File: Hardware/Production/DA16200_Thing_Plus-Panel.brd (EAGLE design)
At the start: 112.3 x 207 mm, 1530 parts, among them J1 Qwiic, J10 CORTEX_JTAG_DEBUG_PTH_NS, J11 Qwiic, J13 USB C, J14 THING_PLUS, J15 CORTEX_JTAG_DEBUG_PTH_NS, J16 Qwiic, J18 USB C, J19 THING_PLUS, J2 THING_PLUS, J20 CORTEX_JTAG_DEBUG_PTH_NS, J21 Qwiic, J23 USB C, J24 THING_PLUS, J25 CORTEX_JTAG_DEBUG_PTH_NS, J26 Qwiic, J28 USB C, J29 THING_PLUS, J3 Qwiic, J30 CORTEX_JTAG_DEBUG_PTH_NS, J31 Qwiic, J33 USB C, J34 THING_PLUS, J35 CORTEX_JTAG_DEBUG_PTH_NS, J36 Qwiic, J38 USB C, J39 THING_PLUS, J40 CORTEX_JTAG_DEBUG_PTH_NS, J41 Qwiic, J43 USB C, J44 THING_PLUS, J45 CORTEX_JTAG_DEBUG_PTH_NS, J46 Qwiic, J48 USB C, J49 THING_PLUS, J5 USB C, J50 CORTEX_JTAG_DEBUG_PTH_NS, J51 Qwiic, J53 USB C, J54 THING_PLUS, J55 CORTEX_JTAG_DEBUG_PTH_NS, J56 Qwiic, J58 USB C, J59 THING_PLUS, J60 CORTEX_JTAG_DEBUG_PTH_NS, J7 CORTEX_JTAG_DEBUG_PTH_NS, J8 USB C, J9 THING_PLUS, Q1 20V/4.2A/52mΩ/1.4W, Q10 20V/4.2A/52mΩ/1.4W, Q11 20V/4.2A/52mΩ/1.4W, Q12 20V/4.2A/52mΩ/1.4W, Q2 20V/4.2A/52mΩ/1.4W, Q3 20V/4.2A/52mΩ/1.4W, Q4 20V/4.2A/52mΩ/1.4W, Q5 20V/4.2A/52mΩ/1.4W, Q6 20V/4.2A/52mΩ/1.4W, Q7 20V/4.2A/52mΩ/1.4W, Q8 20V/4.2A/52mΩ/1.4W, Q9 20V/4.2A/52mΩ/1.4W, U1 DA16200MOD, U10 MCP73831, U11 DA16200MOD, U12 CH340E_MSOP10, U13 XC6222B331MR-G, U14 MCP73831, U15 DA16200MOD, U16 CH340E_MSOP10, U17 XC6222B331MR-G, U18 MCP73831, U19 DA16200MOD, U2 CH340E_MSOP10, U20 CH340E_MSOP10, U21 XC6222B331MR-G, U22 MCP73831, U23 DA16200MOD, U24 CH340E_MSOP10, U25 XC6222B331MR-G, U26 MCP73831, U27 DA16200MOD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

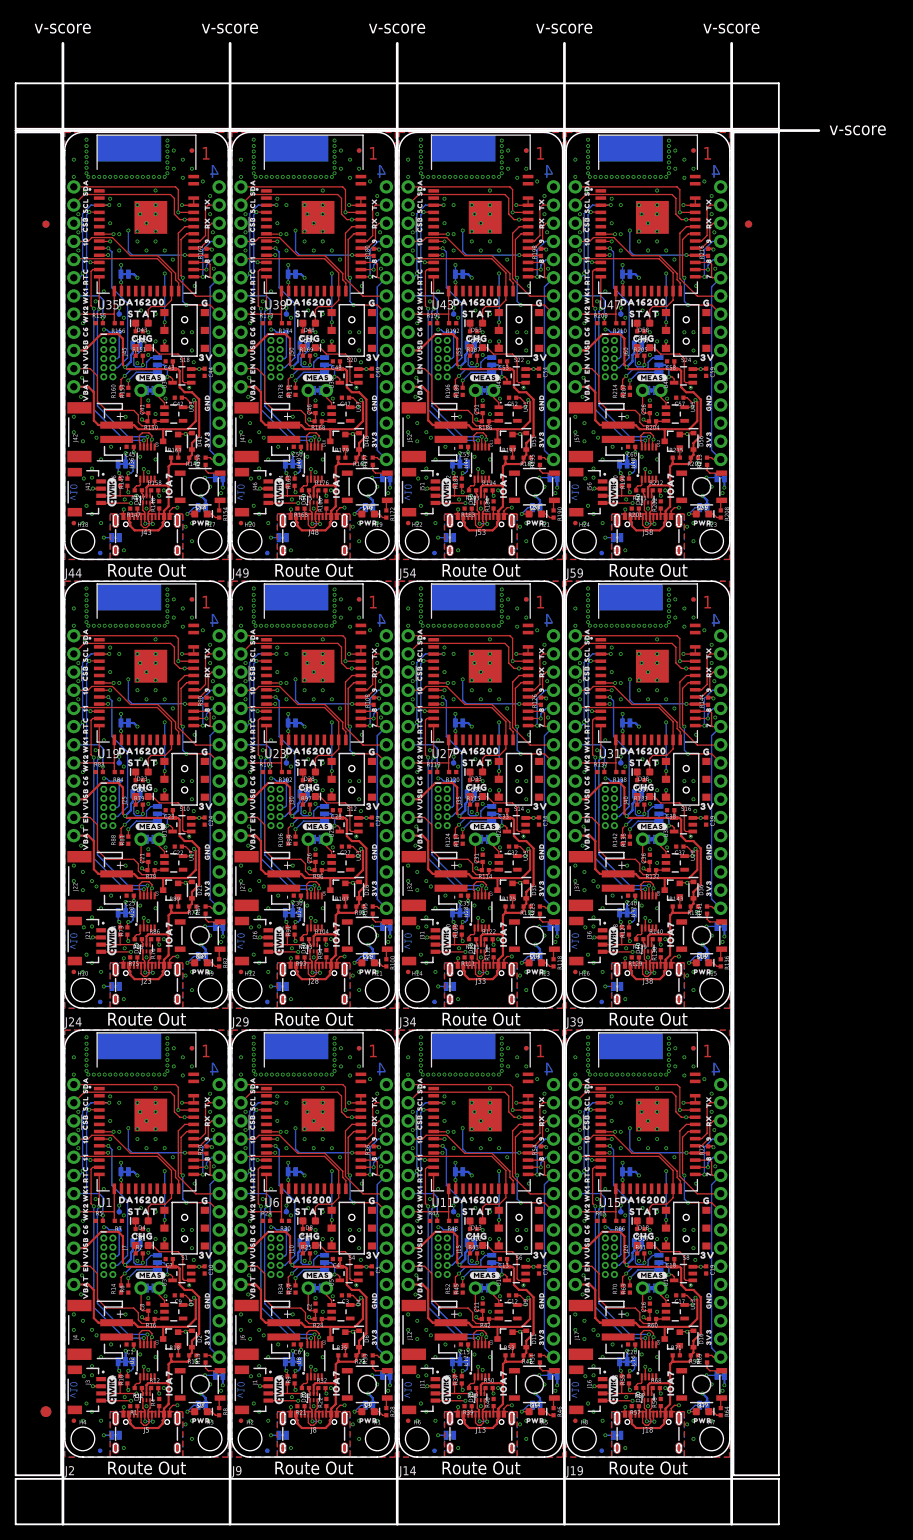
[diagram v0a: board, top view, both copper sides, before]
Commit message: Update production files
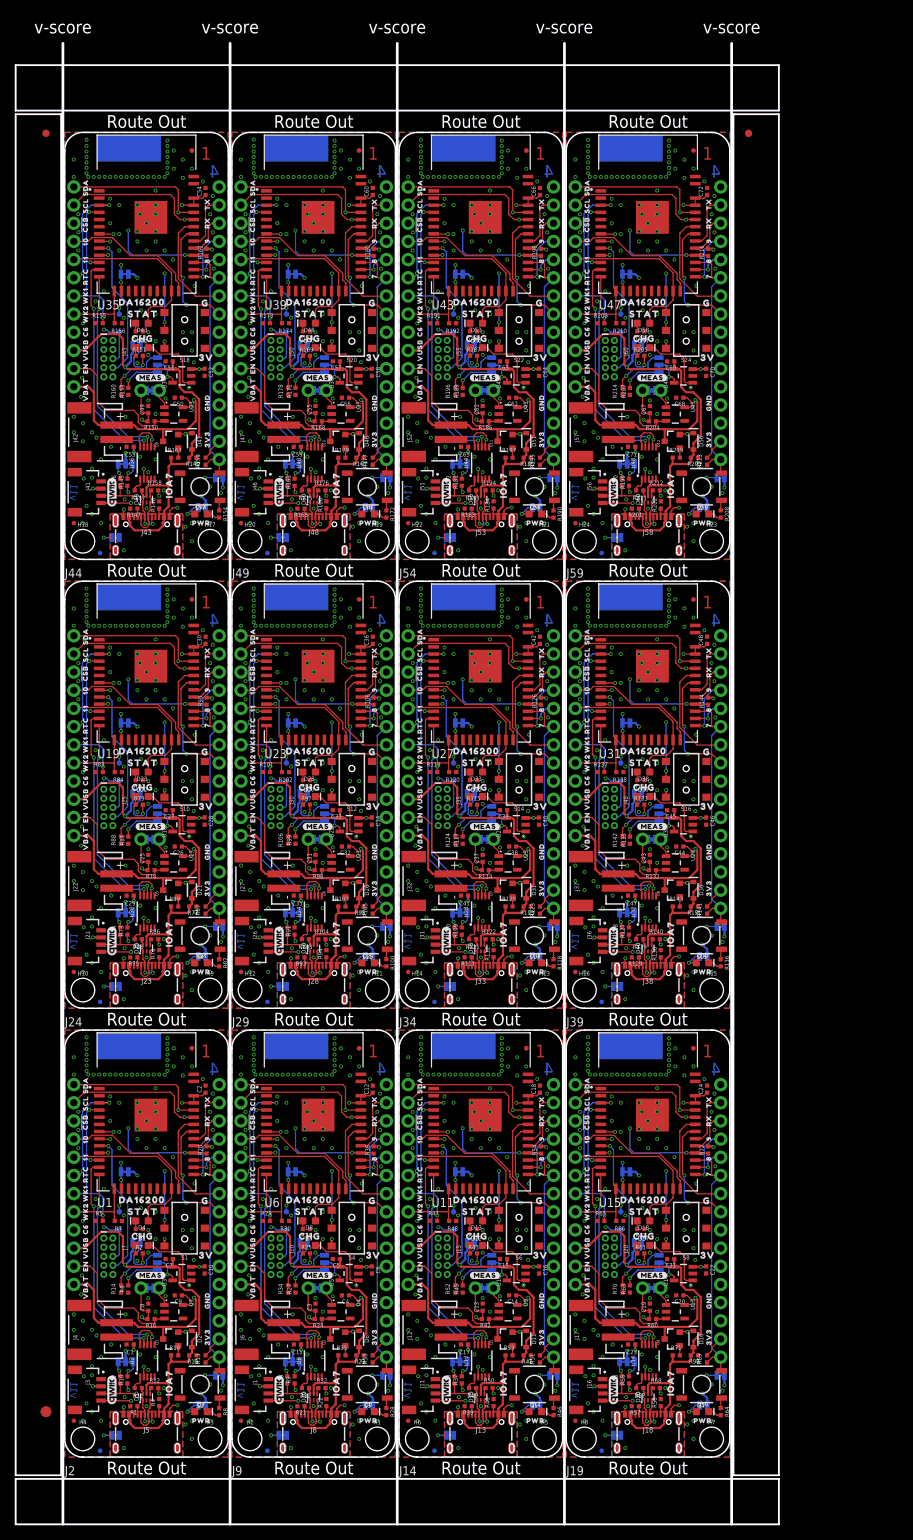
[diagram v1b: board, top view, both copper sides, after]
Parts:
- added C61, C67: 1.0uF, SparkFun-Capacitors:0402-TIGHT
- added C62, C68: 2.2uF, SparkFun-Capacitors:0402-TIGHT
- added C63, C64, C69, C70: 4.7uF, SparkFun-Capacitors:0402-TIGHT
- added C65, C66, C71, C72: 0.1uF, SparkFun-Capacitors:0402-TIGHT
- C11, C2, C36, C41: value 1.0uF -> 0.1uF
- C12, C17, C42, C47: value 2.2uF -> 0.1uF
- C13, C19, C43, C49: value 4.7uF -> 1.0uF
- C14, C38, C4, C44: value 4.7uF -> 2.2uF
- C15, C40, C45, C6: value 0.1uF -> 4.7uF
- C16, C21, C46, C51: value 1.0uF -> 4.7uF
- C18, C23, C24, C29, C48, C53, C54, C59: value 4.7uF -> 0.1uF
- C20, C50: value 0.1uF -> 2.2uF
- C22, C27, C52, C57: value 2.2uF -> 4.7uF
- C25, C55: value 0.1uF -> 1.0uF
- C26, C56: value 1.0uF -> 2.2uF
- C3, C37: value 2.2uF -> 1.0uF
- R105, R123, R13, R141, R159, R177, R195, R213, R33, R51, R69, R87: value 200 -> 10k
- moved C23 98.8 mm to (79.2, 15.7)
- moved C43 96.6 mm to (81.8, 83.7), turned to 90 degrees
- moved C22 94.6 mm to (89.7, 26.2), turned to 270 degrees
- moved C44 93.8 mm to (86.0, 85.3), turned to 180 degrees
- moved C21 92.0 mm to (84.7, 27.7), turned to 180 degrees
- moved C45 91.1 mm to (84.7, 90.4)
- moved C41 81.1 mm to (55.9, 78.5), turned to 180 degrees
- moved C47 80.3 mm to (79.2, 78.5)
- moved C24 79.6 mm to (89.8, 51.4), turned to 90 degrees
- moved C46 79.3 mm to (89.7, 88.9), turned to 270 degrees
- moved C48 64.8 mm to (89.8, 114.2), turned to 90 degrees
- moved C42 60.9 mm to (66.4, 114.2), turned to 90 degrees
- moved C59 58.1 mm to (32.5, 141.2), turned to 180 degrees
- moved C53 53.5 mm to (9.14, 141.2)
- moved C54 53.0 mm to (19.7, 176.9), turned to 90 degrees
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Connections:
- removed net N$107 (its old number): DA_MEAS3.1, U15.15, U15.34, U15.35
- removed net N$117 (its old number): C21.1, D21.C, MEAS4.1, MEAS4.3, Q5.2, R78.2
- removed net N$126 (its old number): R87.1, S9.3
- removed net N$134 (its old number): DA_MEAS4.1, U19.15, U19.34, U19.35
- removed net N$144 (its old number): C26.1, D26.C, MEAS5.1, MEAS5.3, Q6.2, R96.2
- removed net N$153: R105.1, S11.3
- removed net N$161 (its old number): DA_MEAS5.1, U23.15, U23.34, U23.35
- removed net N$171 (its old number): C31.1, D31.C, MEAS6.1, MEAS6.3, Q7.2, R114.2
- removed net N$180 (its old number): R123.1, S13.3
- removed net N$188 (its old number): DA_MEAS6.1, U27.15, U27.34, U27.35
- removed net N$198 (its old number): C36.1, D36.C, MEAS7.1, MEAS7.3, Q8.2, R132.2
- removed net N$215 (its old number): DA_MEAS7.1, U31.15, U31.34, U31.35
- removed net N$225 (its old number): C41.1, D41.C, MEAS8.1, MEAS8.3, Q9.2, R150.2
- removed net N$234 (its old number): R159.1, S17.3
- removed net N$242 (its old number): DA_MEAS8.1, U35.15, U35.34, U35.35
- removed net N$252 (its old number): C46.1, D46.C, MEAS9.1, MEAS9.3, Q10.2, R168.2
- removed net N$261 (its old number): R177.1, S19.3
- removed net N$279 (its old number): C51.1, D51.C, MEAS10.1, MEAS10.3, Q11.2, R186.2
- removed net N$288 (its old number): R195.1, S21.3
- removed net N$296 (its old number): DA_MEAS10.1, U43.15, U43.34, U43.35
- removed net N$306 (its old number): C56.1, D56.C, MEAS11.1, MEAS11.3, Q12.2, R204.2
- removed net N$315: R213.1, S23.3
- removed net N$323: DA_MEAS11.1, U47.15, U47.34, U47.35
- removed net N$36 (its old number): C2.1, D6.C, MEAS1.1, MEAS1.3, Q2.2, R24.2
- removed net N$45 (its old number): R33.1, S3.3
- removed net N$53 (its old number): DA_MEAS1.1, U6.15, U6.34, U6.35
- removed net N$63 (its old number): C11.1, D11.C, MEAS2.1, MEAS2.3, Q3.2, R42.2
- removed net N$72 (its old number): R51.1, S5.3
- removed net N$8 (its old number): R13.1, S2.3
- removed net N$80 (its old number): DA_MEAS2.1, U11.15, U11.34, U11.35
- removed net N$90 (its old number): C16.1, D16.C, MEAS3.1, MEAS3.3, Q4.2, R60.2
- removed net N$99 (its old number): R69.1, S7.3
- new net N$103: C24.1, DA_MEAS3.1, U15.15, U15.34, U15.35
- new net N$113: C25.1, D21.C, MEAS4.1, MEAS4.3, Q5.2, R78.2
- new net N$129: C30.1, DA_MEAS4.1, U19.15, U19.34, U19.35
- new net N$139: C31.1, D26.C, MEAS5.1, MEAS5.3, Q6.2, R96.2
- new net N$155: C36.1, DA_MEAS5.1, U23.15, U23.34, U23.35
- new net N$165: C37.1, D31.C, MEAS6.1, MEAS6.3, Q7.2, R114.2
- new net N$181: C42.1, DA_MEAS6.1, U27.15, U27.34, U27.35
- new net N$191: C43.1, D36.C, MEAS7.1, MEAS7.3, Q8.2, R132.2
- new net N$217: C49.1, D41.C, MEAS8.1, MEAS8.3, Q9.2, R150.2
- new net N$233: C54.1, DA_MEAS8.1, U35.15, U35.34, U35.35
- new net N$243: C55.1, D46.C, MEAS9.1, MEAS9.3, Q10.2, R168.2
- new net N$259: C60.1, DA_MEAS9.1, U39.15, U39.34, U39.35
- new net N$285: C66.1, DA_MEAS10.1, U43.15, U43.34, U43.35
- new net N$295: C67.1, D56.C, MEAS11.1, MEAS11.3, Q12.2, R204.2
- new net N$311: C72.1, DA_MEAS11.1, U47.15, U47.34, U47.35
- new net N$35: C3.1, D6.C, MEAS1.1, MEAS1.3, Q2.2, R24.2
- new net N$51: C12.1, DA_MEAS1.1, U6.15, U6.34, U6.35
- new net N$61: C13.1, D11.C, MEAS2.1, MEAS2.3, Q3.2, R42.2
- new net N$77: C18.1, DA_MEAS2.1, U11.15, U11.34, U11.35
- new net N$87: C19.1, D16.C, MEAS3.1, MEAS3.3, Q4.2, R60.2
- net !RESET!/SPI_CLK: now also R13.1, S2.3; no longer R13.2
- net !RESET!/SPI_CLK1: now also R33.1, S3.3; no longer R33.2
- net !RESET!/SPI_CLK10: now also R195.1, S21.3; no longer R195.2
- net !RESET!/SPI_CLK11: now also R213.1, S23.3; no longer R213.2
- net !RESET!/SPI_CLK2: now also R51.1, S5.3; no longer R51.2
- net !RESET!/SPI_CLK3: now also R69.1, S7.3; no longer R69.2
- net !RESET!/SPI_CLK4: now also R87.1, S9.3; no longer R87.2
- net !RESET!/SPI_CLK5: now also R105.1, S11.3; no longer R105.2
- net !RESET!/SPI_CLK6: now also R123.1, S13.3; no longer R123.2
- net !RESET!/SPI_CLK7: now also R141.1, S15.3; no longer R141.2
- net !RESET!/SPI_CLK8: now also R159.1, S17.3; no longer R159.2
- net !RESET!/SPI_CLK9: now also R177.1, S19.3; no longer R177.2
- net 3.3V: now also R13.2
- net 3.3V1: now also C11.1, C4.1, R33.2; no longer C3.1, C6.1
- net 3.3V10: now also C62.1, C65.1, R195.2; no longer C52.1, C55.1
- net 3.3V11: now also C68.1, C71.1, R213.2; no longer C57.1, C60.1
- net 3.3V2: now also C14.1, C17.1, R51.2; no longer C12.1, C15.1
- net 3.3V3: now also C23.1, R69.2; no longer C17.1
- net 3.3V4: now also C26.1, C29.1, R87.2; no longer C22.1, C25.1
- net 3.3V5: now also C32.1, C35.1, R105.2; no longer C27.1, C30.1
- net 3.3V6: now also C38.1, C41.1, R123.2; no longer C32.1, C35.1
- net 3.3V7: now also C44.1, C47.1, R141.2; no longer C37.1, C40.1
- net 3.3V8: now also C50.1, C53.1, R159.2; no longer C42.1, C45.1
- net 3.3V9: now also C56.1, C59.1, R177.2; no longer C47.1, C50.1
- net GND: now also C2.2
- net GND1: now also C11.2, C12.2; no longer C2.2
- net GND10: now also C61.2, C62.2, C63.2, C64.2, C65.2, C66.2; no longer C51.2, C52.2, C53.2, C54.2, C55.2
- net GND11: now also C67.2, C68.2, C69.2, C70.2, C71.2, C72.2; no longer C56.2, C57.2, C58.2, C59.2, C60.2
- net GND2: now also C16.2, C17.2, C18.2; no longer C11.2, C12.2
- net GND3: now also C21.2, C22.2, C23.2, C24.2; no longer C16.2, C17.2, C18.2
- net GND4: now also C26.2, C27.2, C28.2, C29.2, C30.2; no longer C21.2, C22.2, C23.2, C24.2
- net GND5: now also C31.2, C32.2, C33.2, C34.2, C35.2, C36.2; no longer C26.2, C27.2, C28.2, C29.2, C30.2
- net GND6: now also C37.2, C38.2, C39.2, C40.2, C41.2, C42.2; no longer C31.2, C32.2, C33.2, C34.2, C35.2
- net GND7: now also C43.2, C44.2, C45.2, C46.2, C47.2, C48.2; no longer C36.2, C37.2, C38.2, C39.2, C40.2
- net GND8: now also C49.2, C50.2, C51.2, C52.2, C53.2, C54.2; no longer C41.2, C42.2, C43.2, C44.2, C45.2
- net GND9: now also C55.2, C56.2, C57.2, C58.2, C59.2, C60.2; no longer C46.2, C47.2, C48.2, C49.2, C50.2
- net N$207: now also C48.1, DA_MEAS7.1, U31.15, U31.34, U31.35; no longer R141.1, S15.3
- net N$25: now also C2.1
- net N$269: now also C61.1, D51.C, MEAS10.1, MEAS10.3, Q11.2, R186.2; no longer DA_MEAS9.1, U39.15, U39.34, U39.35
- net V_BATT1: now also C6.1; no longer C5.1
- net V_BATT10: now also C64.1; no longer C54.1
- net V_BATT11: now also C70.1; no longer C59.1
- net V_BATT2: now also C16.1; no longer C14.1
- net V_BATT3: now also C22.1; no longer C19.1
- net V_BATT4: now also C28.1; no longer C24.1
- net V_BATT5: now also C34.1; no longer C29.1
- net V_BATT6: now also C40.1; no longer C34.1
- net V_BATT7: now also C46.1; no longer C39.1
- net V_BATT8: now also C52.1; no longer C44.1
- net V_BATT9: now also C58.1; no longer C49.1
- net V_USB1: now also C5.1; no longer C4.1
- net V_USB10: now also C63.1; no longer C53.1
- net V_USB11: now also C69.1; no longer C58.1
- net V_USB2: now also C15.1; no longer C13.1
- net V_USB3: now also C21.1; no longer C18.1
- net V_USB4: now also C27.1; no longer C23.1
- net V_USB5: now also C33.1; no longer C28.1
- net V_USB6: now also C39.1; no longer C33.1
- net V_USB7: now also C45.1; no longer C38.1
- net V_USB8: now also C51.1; no longer C43.1
- net V_USB9: now also C57.1; no longer C48.1
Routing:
- net N$311: track 0.00 -> 24.0 mm, vias 0 -> 3
- net N$233: track 0.00 -> 24.0 mm, vias 0 -> 3
- net N$285: track 0.00 -> 24.0 mm, vias 0 -> 3
- net N$259: track 0.00 -> 24.0 mm, vias 0 -> 3
- net N$103: track 0.00 -> 24.0 mm, vias 0 -> 3
- net N$77: track 0.00 -> 24.0 mm, vias 0 -> 3
- net N$51: track 0.00 -> 24.0 mm, vias 1 -> 3
- net N$181: track 0.00 -> 24.0 mm, vias 0 -> 3
- net N$129: track 0.00 -> 24.0 mm, vias 0 -> 3
- net N$155: track 0.00 -> 24.0 mm, vias 0 -> 3
- net N$323: track 22.2 -> 0.00 mm, vias 3 -> 0
- net N$296 (its old number): track 22.2 -> 0.00 mm, vias 3 -> 0
- net N$242 (its old number): track 22.2 -> 0.00 mm, vias 3 -> 0
- net N$107 (its old number): track 22.2 -> 0.00 mm, vias 3 -> 0
- net N$80 (its old number): track 22.2 -> 0.00 mm, vias 3 -> 0
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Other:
- board size 112.3 x 207 mm -> 106.7 x 207 mm
- board text added: "v11"
- board text removed: "v10"
